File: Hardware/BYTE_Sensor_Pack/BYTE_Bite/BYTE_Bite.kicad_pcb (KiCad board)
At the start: 2 copper layers, 12.2 x 9 mm, 1 part, among them J1 Bite

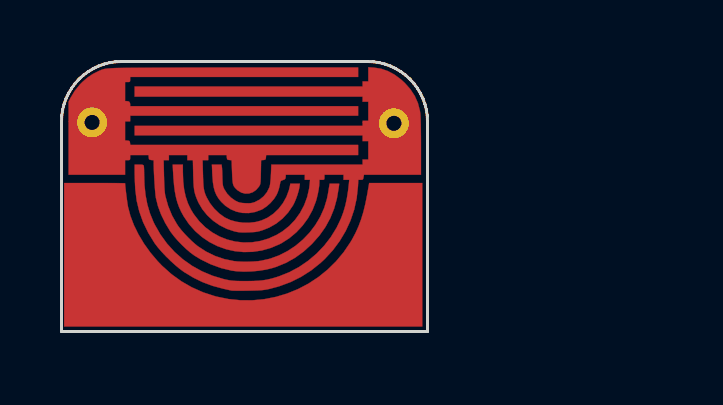
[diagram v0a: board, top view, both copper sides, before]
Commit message: add projects
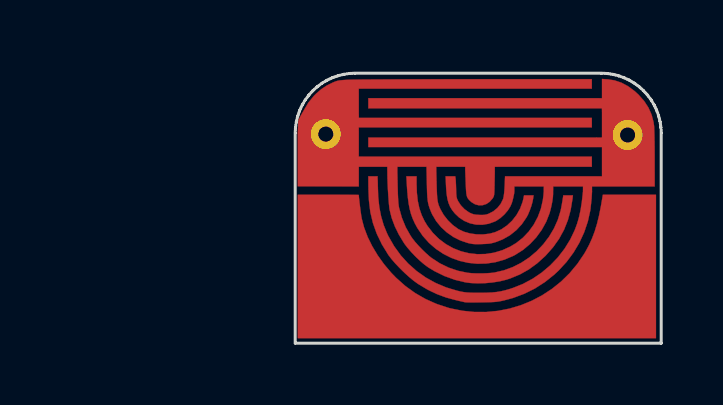
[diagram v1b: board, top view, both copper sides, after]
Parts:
- moved J1 7.80 mm to (156.0, 82.9)
